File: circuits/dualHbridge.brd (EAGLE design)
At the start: 76.2 x 76.8 mm, 43 parts, among them Q1 FDS5680, Q2 FDS5680, Q3 FDS5680, Q4 FDS5680, Q5 FDS5680, Q6 FDS5680, Q7 FDS5680, Q8 FDS5680

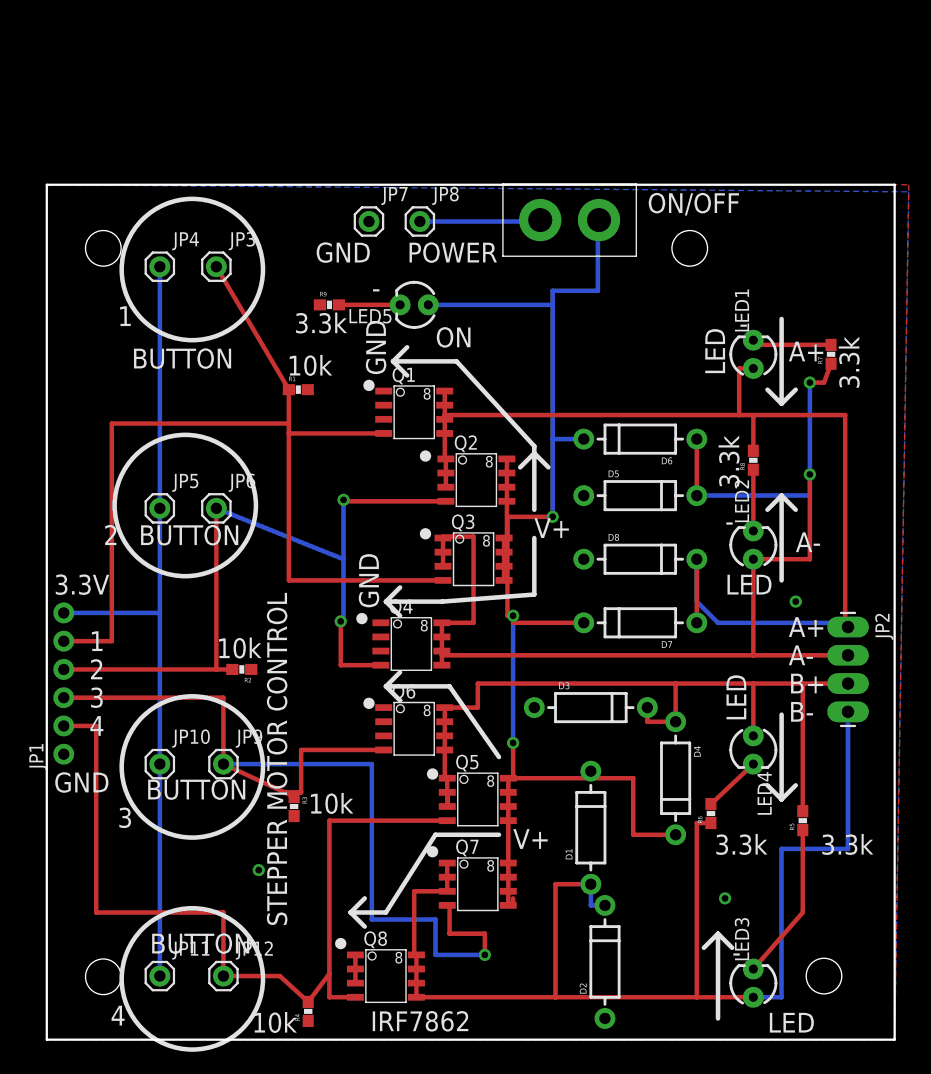
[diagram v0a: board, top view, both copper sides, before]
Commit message: h bridge circuit board
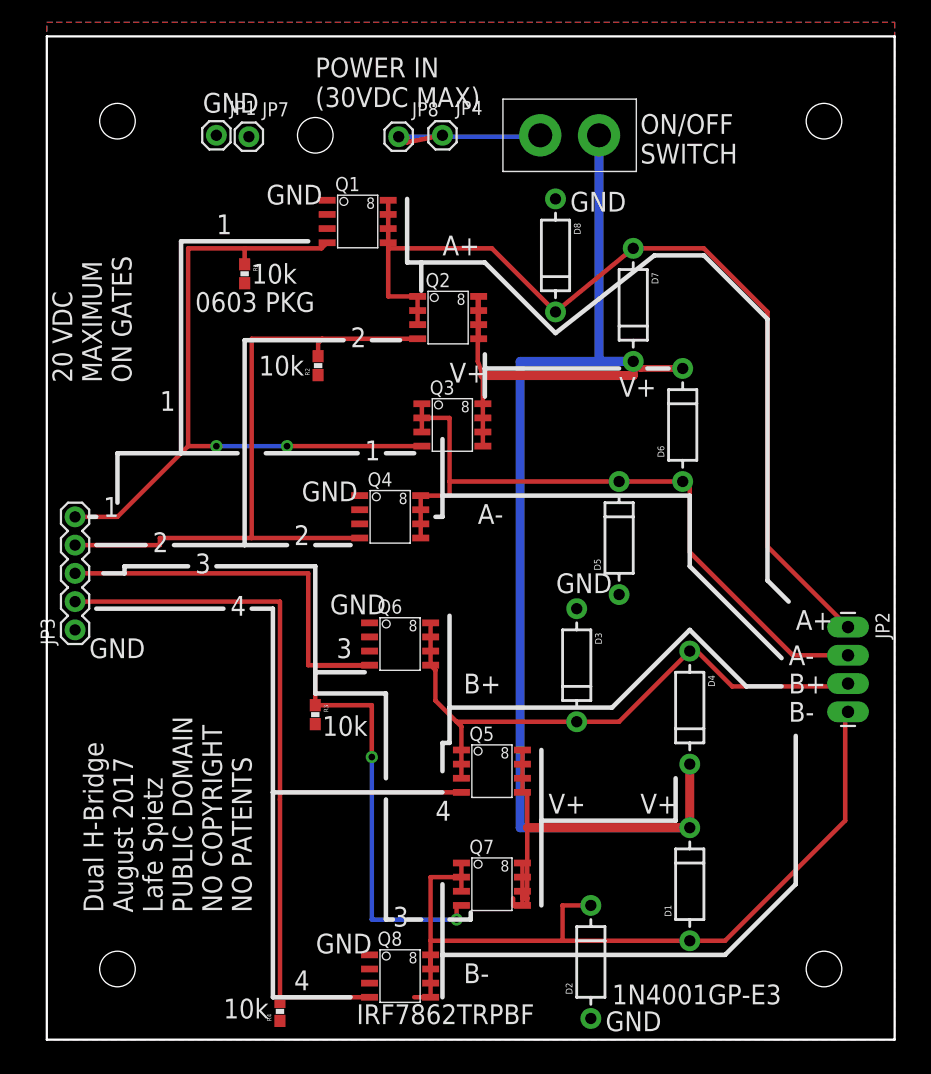
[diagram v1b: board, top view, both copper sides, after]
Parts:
- removed JP10, JP11, JP12, JP5, JP6, JP9: M01PTH, SparkFun-Connectors:1X01
- removed LED1, LED2, LED3, LED4, LED5: (no value), SparkFun-LED:LED3MM
- removed R5, R6, R7, R8, R9: 3.3k, SparkFun-Passives:0603-RES
- JP1: value (none) -> M01PTH; device SparkFun-Connectors:1X06_NO_SILK -> SparkFun-Connectors:1X01
- JP3: value M01PTH -> (none); device SparkFun-Connectors:1X01 -> SparkFun-Connectors:1X05
- moved JP1 57.3 mm to (15.2, 81.3), turned to 0 degrees
- moved JP3 35.0 mm to (2.54, 36.8), turned to 90 degrees
- moved D7 28.6 mm to (52.7, 66.0), turned to 270 degrees
- moved D8 28.3 mm to (45.7, 70.5), turned to 270 degrees
- moved R2 28.2 mm to (24.4, 60.6), turned to 90 degrees
- moved JP4 28.0 mm to (35.6, 81.3)
- moved Q1 17.9 mm to (27.9, 73.5)
- moved Q2 14.8 mm to (36.1, 64.9)
- moved JP7 13.2 mm to (18.2, 81.2)
- moved Q3 12.2 mm to (36.4, 55.2)
- moved Q4 11.6 mm to (30.9, 47.0)
- moved R1 11.5 mm to (17.8, 68.8), turned to 270 degrees
- moved D1 10.2 mm to (57.8, 14.0)
- moved R3 8.47 mm to (24.1, 29.2)
- moved JP8 7.85 mm to (31.6, 81.2)
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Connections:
- removed net N$1: LED1.K, R7.2
- removed net N$10: LED4.K, R6.2
- removed net N$16: LED5.K, R9.2
- removed net N$8: LED2.K, R8.1
- removed net N$9: LED3.K, R5.1
- removed net V3.3: JP1.6, JP10.1, JP11.1, JP4.1, JP5.1
- net 12V: no longer LED5.A
- net A+: no longer LED1.A, R8.2
- net A-: no longer LED2.A, R7.1
- net B+: no longer LED4.A, R5.2
- net B-: no longer LED3.A, R6.1
- net GND: now also JP3.1; no longer R9.1
- net N$13: now also JP3.3; no longer JP1.3, JP9.1
- net N$14: now also JP3.2; no longer JP1.2, JP12.1
- net N$15: now also JP4.1
- net N$6: now also JP3.5; no longer JP1.5, JP3.1
- net N$7: now also JP3.4; no longer JP1.4, JP6.1
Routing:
- net V3.3: track 72.4 -> 0.00 mm
- net 12V: track 125.0 -> 169.3 mm, vias 3 -> 0
- net A-: track 106.1 -> 64.0 mm, vias 2 -> 0
- net B-: track 113.3 -> 76.2 mm
- net N$6: track 92.1 -> 65.7 mm, vias 0 -> 2
- net B+: track 72.2 -> 54.3 mm
- net N$9: track 14.2 -> 0.00 mm
- net N$13: track 88.5 -> 76.9 mm, vias 1 -> 2
- net A+: track 97.0 -> 86.0 mm
- net N$7: track 70.0 -> 60.8 mm, vias 2 -> 0
- net N$1: track 7.41 -> 0.00 mm
- net N$15: track 10.9 -> 17.4 mm
- net N$8: track 5.50 -> 0.00 mm
- net N$16: track 5.50 -> 0.00 mm
- net N$10: track 5.24 -> 0.00 mm
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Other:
- board size 76.2 x 76.8 mm -> 76.2 x 90.2 mm
- board text added: "0603 PKG"
- board text added: "1N4001GP-E3"
- board text added: "20 VDC MAXIMUM ON GATES"
- board text added: "Dual H-Bridge August 2017 Lafe Spietz PUBLIC DOMAIN NO COPYRIGHT NO PATENTS"
- board text added: "IRF7862TRPBF"
- board text added: "ON/OFF SWITCH"
- board text added: "POWER IN (30VDC MAX)"
- board text added: "Vin"
- board text removed: "-"
- board text removed: "3.3V"
- board text removed: "3.3k"
- board text removed: "BUTTON"
- board text removed: "IRF7862"
- board text removed: "LED"
- board text removed: "NO PATENTS NO COPYRIGHTS NO MONEY NO MINING NO PROPERTY"
- board text removed: "ON"
- board text removed: "ON/OFF"
- board text removed: "POWER"
- board text removed: "STEPPER MOTOR CONTROL"
